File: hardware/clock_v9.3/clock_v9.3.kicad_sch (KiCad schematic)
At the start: 89 parts, among them J4 USB_C_Receptacle, J8 Conn_01x02, U1 SN74LVC1G14DBV, U11 AMS1117-3.3, U12 BA50DD0WHFP-TR, U14 CH340C, U15 USBLC6-2P6, U2 SN74LVC1G14DBV, U23 TPS63060, U3 SN74LVC1G14DBV, U4 LM2731XMF, U9 L78L05_SOT89

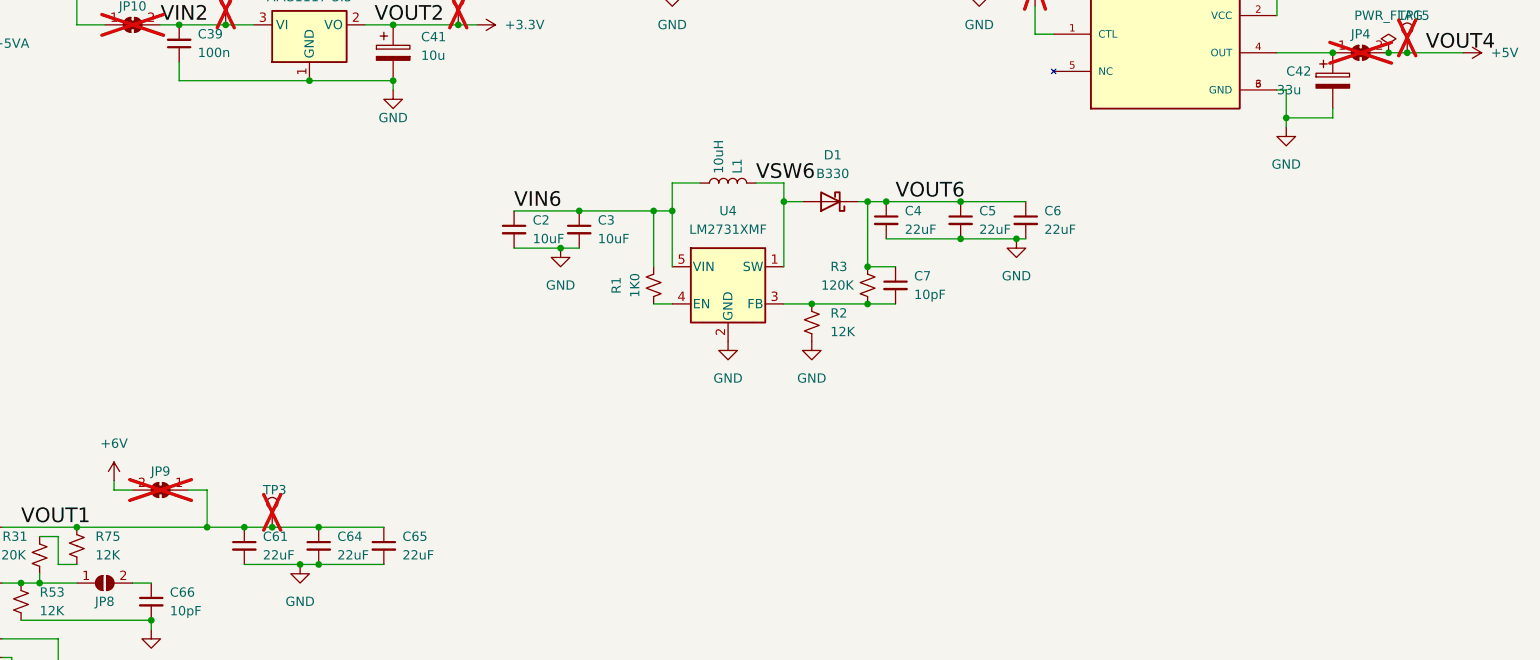
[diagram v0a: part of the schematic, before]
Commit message: start 2nd supply
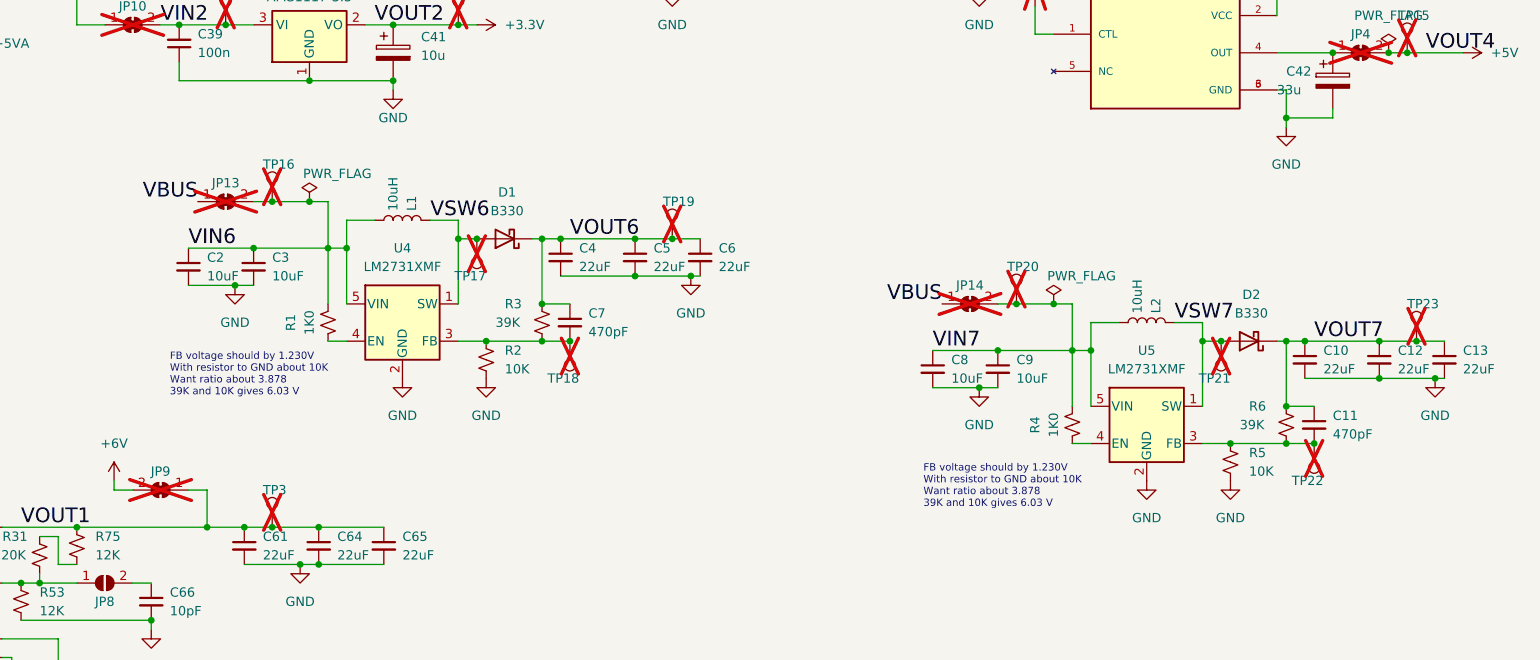
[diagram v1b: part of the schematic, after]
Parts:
- added C10, C12, C13: 22uF, Capacitor_SMD:C_0805_2012Metric, symbol Device:C_Small
- added C11: 470pF, Capacitor_SMD:C_0603_1608Metric, symbol Device:C_Small
- added C8, C9: 10uF, Capacitor_SMD:C_0603_1608Metric, symbol Device:C_Small
- added D2: B330, Diode_SMD:D_SMC, symbol Diode:B330
- added JP13, JP14: SolderJumper_2_Bridged, Jumper:SolderJumper-2_P1.3mm_Bridged2Bar_RoundedPad1.0x1.5mm, symbol Jumper:SolderJumper_2_Bridged
- added L2: 10uH, Inductor_SMD:L_Coilcraft_XAL4020-XXX, symbol Device:L
- added R4: 1K0, Resistor_SMD:R_0603_1608Metric, symbol Device:R_Small_US
- added R5: 10K, Resistor_SMD:R_0603_1608Metric, symbol Device:R_Small_US
- added R6: 39K, Resistor_SMD:R_0603_1608Metric, symbol Device:R_Small_US
- added TP16, TP17, TP18, TP19, TP20, TP21, TP22, TP23: ~, TestPoint:TestPoint_THTPad_D1.5mm_Drill0.7mm, symbol Connector:TestPoint
- added U5: LM2731XMF, Package_TO_SOT_SMD:SOT-23-5, symbol Regulator_Switching:LM2731XMF
- C7: value 10pF -> 470pF; JLCPCB Part # C1634 -> C1620
- R2: value 12K -> 10K; JLCPCB Part # C22790 -> C25804
- R3: value 120K -> 39K; JLCPCB Part # C25808 -> C23153
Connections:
- net GND: now also C10.2, C12.2, C13.2, C8.2, C9.2, R5.2, U5.2 (GND)
- net VBUS: now also JP13.1 (A), JP14.1 (A)
- net VIN6: now also JP13.2 (B), TP16.1
- net VOUT6: now also TP19.1
- net VSW6: now also TP17.1
- net at C7.2, R2.1, R3.2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: now also TP18.1
- new net: R4.2, U5.4 (EN)
- new net: C11.2, R5.1, R6.2, TP22.1, U5.3 (FB)
- new net VIN7: C8.1, C9.1, JP14.2 (B), L2.2, R4.1, TP20.1, U5.5 (VIN)
- new net VOUT7: C10.1, C11.1, C12.1, C13.1, D2.1 (K), R6.1, TP23.1
- new net VSW7: D2.2 (A), L2.1, TP21.1, U5.1 (SW)
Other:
- note added: "FB voltage should by 1.230V With resistor to GND about 10K Want ratio about 3.878 39K and 10K gives 6.03 V"
- moved on the sheet: C2, C3, C4, C5, C6, C7, D1, L1, R1, R2, R3, U4
